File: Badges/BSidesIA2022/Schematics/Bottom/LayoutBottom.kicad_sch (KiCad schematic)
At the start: 55 parts, among them J1 Program, J10 Cap Sense, J11 Cap Sense, J12 Cap Sense, J13 Cap Sense, J14 Neopixel Expansion, J2 Left_IN, J3 Right_Out, J4 Cap Sense, J5 Conn_01x10, J6 Conn_01x01, J7 Conn_01x01, J8 Conn_01x01, J9 Conn_01x01, P1 USB_C_Plug_corrected, SW1 SW_SPDT, SW2 SW_Push, SW3 SW_Push, SW4 SW_Push, SW5 SW_Push, SW6 SW_Push, U1 HX4055M, U10 SK6812_Side, U2 SK6812_Side, U3 ESP32-S2-SOLO, U4 SK6812_Side, U5 SK6812_Side, U6 SK6812_Side, U7 SK6812_Side, U8 SK6812_Side, U9 SK6812_Side

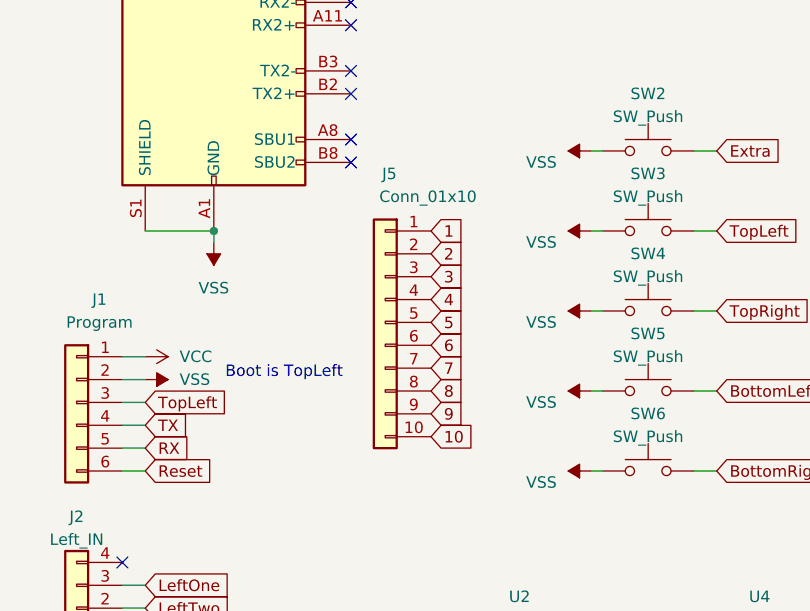
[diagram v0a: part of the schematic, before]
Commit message: Mostly final Corncon
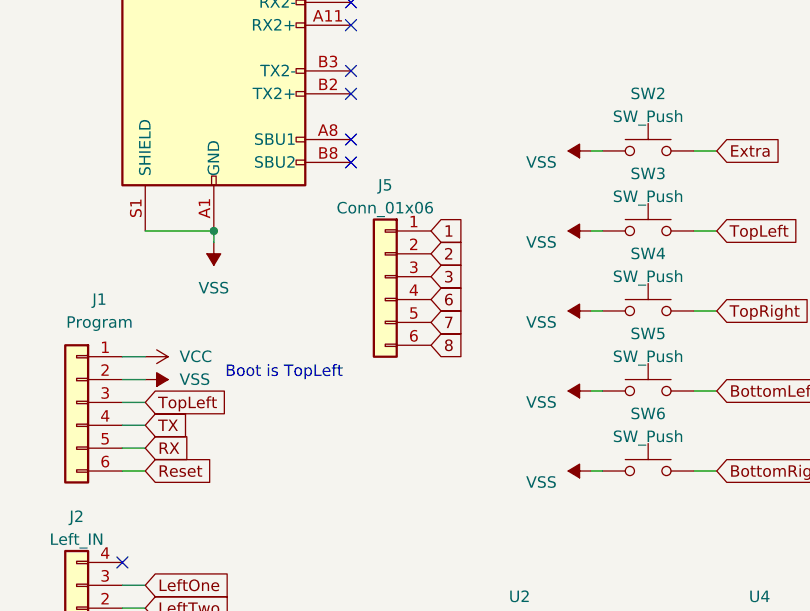
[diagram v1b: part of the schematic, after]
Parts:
- removed J5: Conn_01x10, Connector_PinHeader_2.54mm:PinHeader_1x10_P2.54mm_Vertical, symbol Connector_Generic:Conn_01x10
- added J5: Conn_01x06, Connector_PinHeader_2.54mm:PinHeader_1x06_P2.54mm_Vertical, symbol Connector_Generic:Conn_01x06
- J10, J11, J12, J13: footprint CornConStranger:CapSence -> Bsides22:CapSense
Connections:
- net 1: now also J5.1 (Pin_1)
- net 2: now also J5.2 (Pin_2)
- net 3: now also J5.3 (Pin_3)
- net 6: now also J5.4 (Pin_4)
- net 7: now also J5.5 (Pin_5)
- net 8: now also J5.6 (Pin_6)
